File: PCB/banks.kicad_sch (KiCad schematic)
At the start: 50 parts, among them U1 XC7A50T-FGG484, Y3 100MHz

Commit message: a bunch more routing and assigning, really messy but coming along
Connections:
- net DDR_BA0: now reaches U1.AA4 (IO_L11N_T1_SRCC_34)
- net DDR_A12: now reaches U1.AA8 (IO_L22P_T3_34)
- net DDR_A14: now reaches U1.AB1 (IO_L7N_T1_34)
- net ~{DDR_RESET}: now reaches U1.AB2 (IO_L8N_T1_34)
- net ~{DDR_WE}: now reaches U1.AB3 (IO_L8P_T1_34)
- net DDR_A10: now reaches U1.AB8 (IO_L22N_T3_34)
- net DDR_A9: now reaches U1.R2 (IO_L3N_T0_DQS_34)
- net DDR_A6: now reaches U1.T1 (IO_L1P_T0_34)
- net DDR_BA2: now reaches U1.T3 (IO_0_34)
- net DDR_A1: now reaches U1.U1 (IO_L1N_T0_34)
- net DDR_A4: now reaches U1.U2 (IO_L2P_T0_34)
- net DDR_A5: now reaches U1.U3 (IO_L6P_T0_34)
- net ~{DDR_ODT}: now reaches U1.V3 (IO_L6N_T0_VREF_34)
- net DDR_A11: now reaches U1.W1 (IO_L5P_T0_34)
- net DDR_A7: now reaches U1.W2 (IO_L4P_T0_34)
- net DDR_A3: now reaches U1.W4 (IO_L12N_T1_MRCC_34)
- net DDR_CKE: now reaches U1.W5 (IO_L15N_T2_DQS_34)
- net DDR_DQM1: now reaches U1.W9 (IO_L24P_T3_34)
- net DDR_A13: now reaches U1.Y1 (IO_L5N_T0_34)
- net DDR_A2: now reaches U1.Y2 (IO_L4N_T0_34)
- net DDR_A0: now reaches U1.Y4 (IO_L11P_T1_SRCC_34)
- net ~{DDR_CAS}: now reaches U1.Y6 (IO_L18P_T2_34)
- no-connect marks 10 -> 17
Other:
- moved on the sheet: C149, C152, C153, C154, C155, C156, C157, C158, C159, C160, C161, C162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

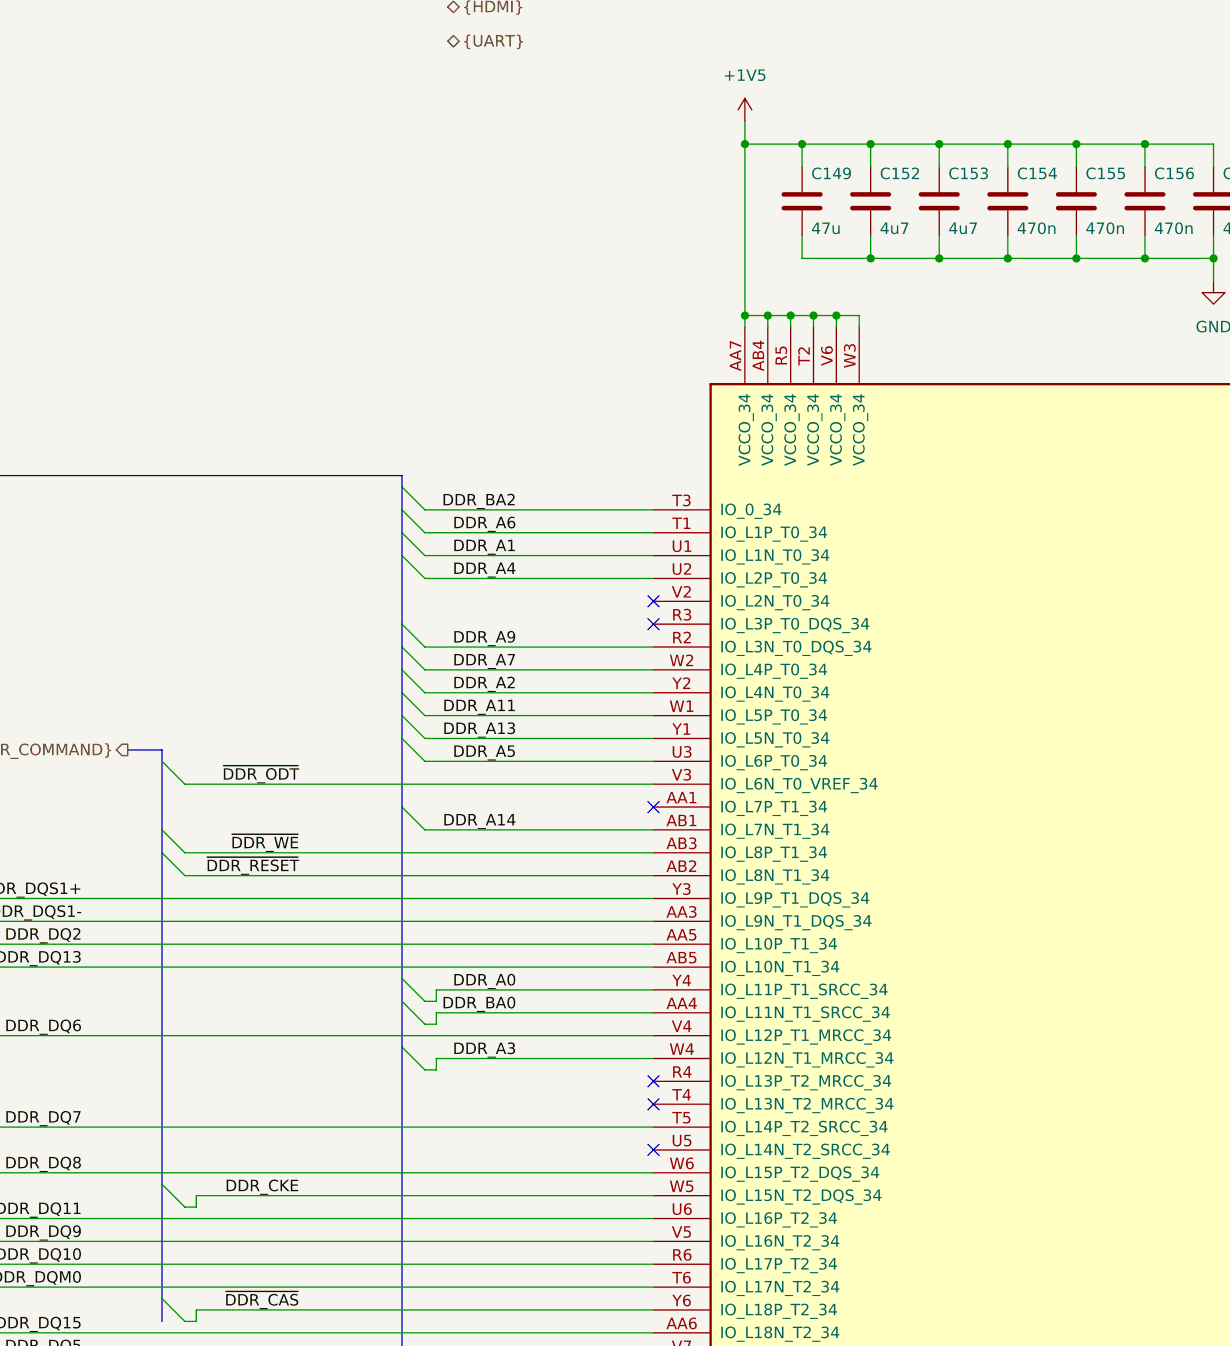
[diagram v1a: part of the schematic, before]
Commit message: finished routing all the pins, very messy still
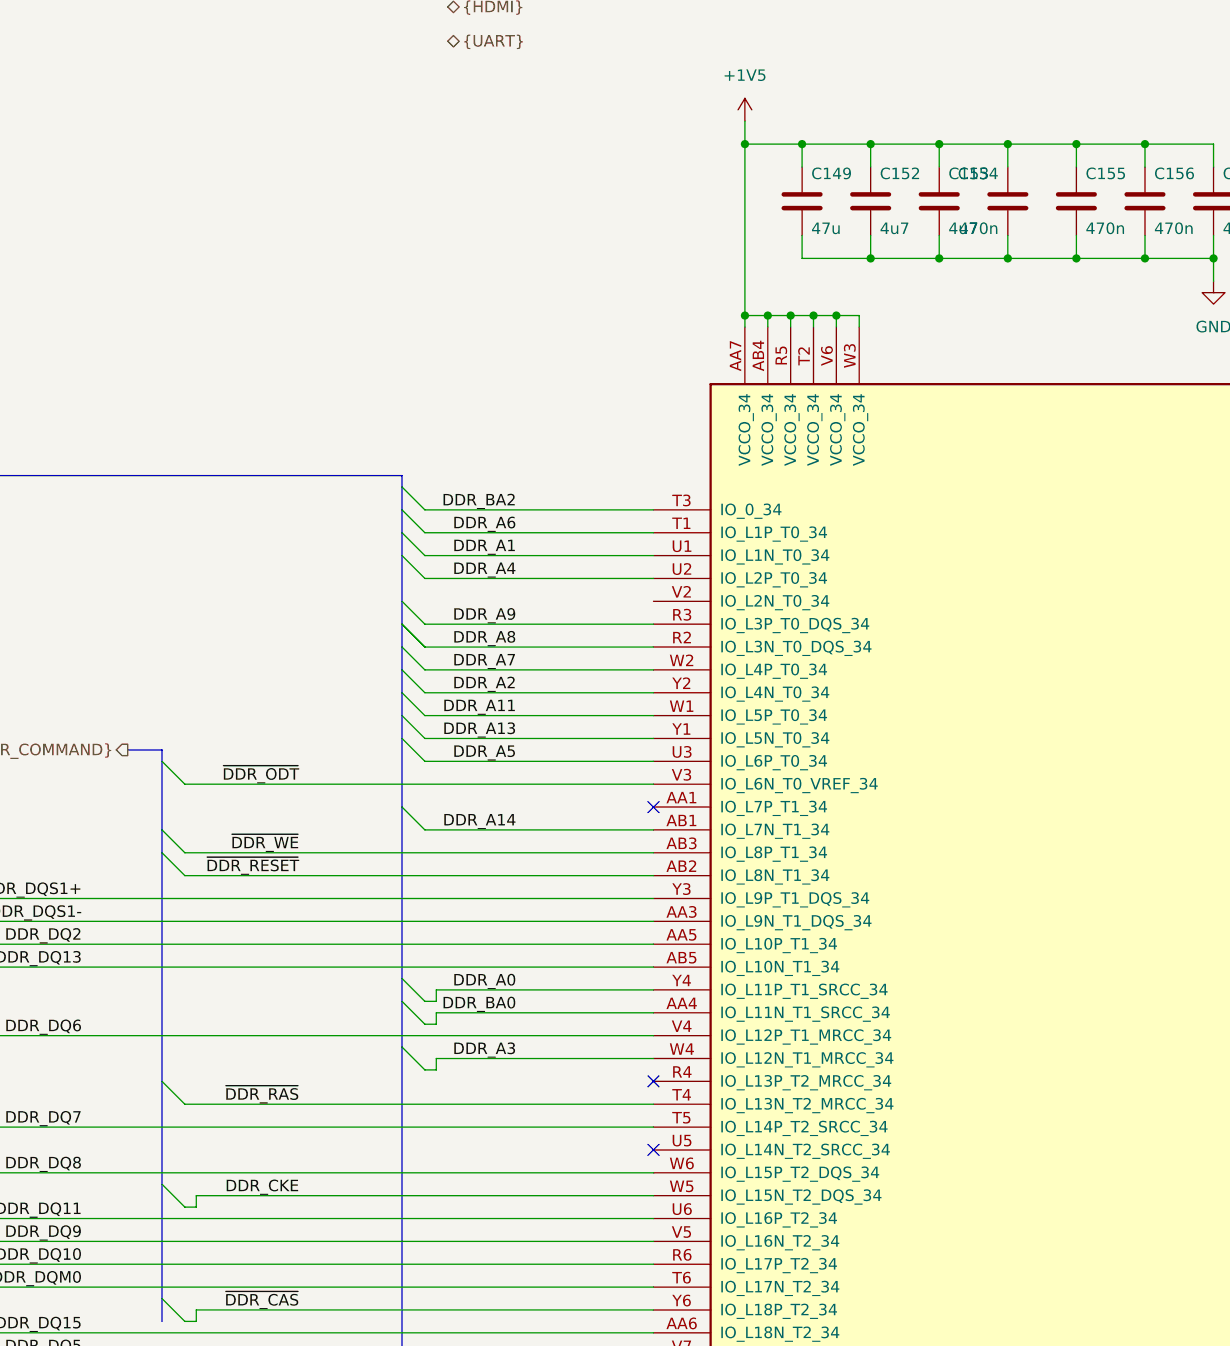
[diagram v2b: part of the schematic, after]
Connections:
- net DDR_A9: now also U1.R3 (IO_L3P_T0_DQS_34); no longer U1.R2 (IO_L3N_T0_DQS_34)
- net ~{DDR_RAS}: now reaches U1.T4 (IO_L13N_T2_MRCC_34)
- new net DDR_A8: U1.R2 (IO_L3N_T0_DQS_34)
- no-connect marks 17 -> 14
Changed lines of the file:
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@@
 	)
 	(no_connect
-		(at 702.31 102.87)
-	)
-	(no_connect
 		(at 261.62 209.55)
 	)
@@
 	)
 	(no_connect
-		(at 702.31 156.21)
-	)
-	(no_connect
 		(at 702.31 214.63)
 	)
@@
 	)
 	(no_connect
-		(at 702.31 100.33)
-	)
-	(no_connect
 		(at 127 113.03)
 	)
@@
 	)
 	(bus_entry
+		(at 647.7 153.67)
+		(size 2.54 2.54)
+		(stroke
+			(width 0)
+			(type default)
+		)
+	)
+	(bus_entry
 		(at 622.3 168.91)
 		(size 2.54 2.54)
@@
 	)
 	(bus_entry
+		(at 674.37 100.33)
+		(size 2.54 2.54)
+		(stroke
+			(width 0)
+			(type default)
+		)
+	)
+	(bus_entry
 		(at 622.3 179.07)
 		(size 2.54 2.54)
@@
 	)
 	(bus_entry
+		(at 674.37 102.87)
+		(size 2.54 2.54)
+		(stroke
+			(width 0)
+			(type default)
+		)
+	)
+	(bus_entry
 		(at 674.37 87.63)
 		(size 2.54 2.54)
@@
 	(bus
 		(pts
-			(xy 674.37 95.25) (xy 674.37 102.87)
+			(xy 674.37 95.25) (xy 674.37 100.33)
 		)
 		(stroke
@@
 		)
 	)
+	(bus
+		(pts
+			(xy 647.7 153.67) (xy 647.7 165.1)
+		)
+		(stroke
+			(width 0)
+			(type default)
+		)
+	)
 	(wire
 		(pts
@@
 	(wire
 		(pts
+			(xy 650.24 156.21) (xy 702.31 156.21)
+		)
+		(stroke
+			(width 0)
+			(type default)
+		)
+	)
+	(wire
+		(pts
 			(xy 125.73 49.53) (xy 125.73 52.07)
 		)
@@
 	(bus
 		(pts
-			(xy 647.7 128.27) (xy 647.7 165.1)
+			(xy 647.7 128.27) (xy 647.7 153.67)
 		)
 		(stroke
@@
 	(wire
 		(pts
+			(xy 676.91 102.87) (xy 702.31 102.87)
+		)
+		(stroke
+			(width 0)
+			(type default)
+		)
+	)
+	(wire
+		(pts
 			(xy 281.94 68.58) (xy 281.94 69.85)
 		)
@@
 		)
 	)
+	(bus
+		(pts
+			(xy 674.37 100.33) (xy 674.37 102.87)
+		)
+		(stroke
+			(width 0)
+			(type default)
+		)
+	)
 	(wire
 		(pts
@@
 		)
 	)
+	(label "~{DDR_RAS}"
+		(at 662.94 156.21 180)
+		(effects
+			(font
+				(size 1.27 1.27)
+			)
+			(justify right bottom)
+		)
+	)
 	(label "DDR_DQS1+"
 		(at 638.81 133.35 180)
@@
 		)
 	)
-	(label "DDR_A9"
-		(at 687.07 105.41 180)
-		(effects
-			(font
-				(size 1.27 1.27)
-			)
-			(justify right bottom)
-		)
-	)
 	(label "~{PCIe_PEWAKE}"
 		(at 175.26 168.91 180)
@@
 		)
 	)
+	(label "DDR_A8"
+		(at 687.07 105.41 180)
+		(effects
+			(font
+				(size 1.27 1.27)
+			)
+			(justify right bottom)
+		)
+	)
 	(label "DDR_DQ4"
 		(at 638.81 186.69 180)
@@
 		)
 	)
+	(label "DDR_A9"
+		(at 687.07 102.87 180)
+		(effects
+			(font
+				(size 1.27 1.27)
+			)
+			(justify right bottom)
+		)
+	)
 	(hierarchical_label "{PCIe_COMMAND}"
 		(shape bidirectional)
@@
 		(lib_id "Device:C")
 		(at 741.68 55.88 0)
+		(mirror y)
 		(unit 1)
 		(exclude_from_sim no)
@@
 		(dnp no)
 		(property "Reference" "C154"
-			(at 742.696 52.832 0)
+			(at 740.664 52.832 0)
 			(effects
 				(font
@@
 		)
 		(property "Value" "470n"
-			(at 742.696 58.928 0)
+			(at 740.664 58.928 0)
 			(effects
 				(font
@@
 		)
 		(property "Footprint" "Capacitor_SMD:C_0201_0603Metric"
-			(at 742.6452 59.69 0)
+			(at 740.7148 59.69 0)
 			(effects
 				(font
